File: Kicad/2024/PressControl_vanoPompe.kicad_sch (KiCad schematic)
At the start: 27 parts, among them J1 Conn_01x08_Pin, J2 Conn_01x08_Socket, J5 Conn_01x08_Socket, J6 Conn_01x08_Pin, K1 sOnOff_ClearContacts, P1 Pump, P2 Press_Control, SW1 TestAlarm, SW2 pc_Button

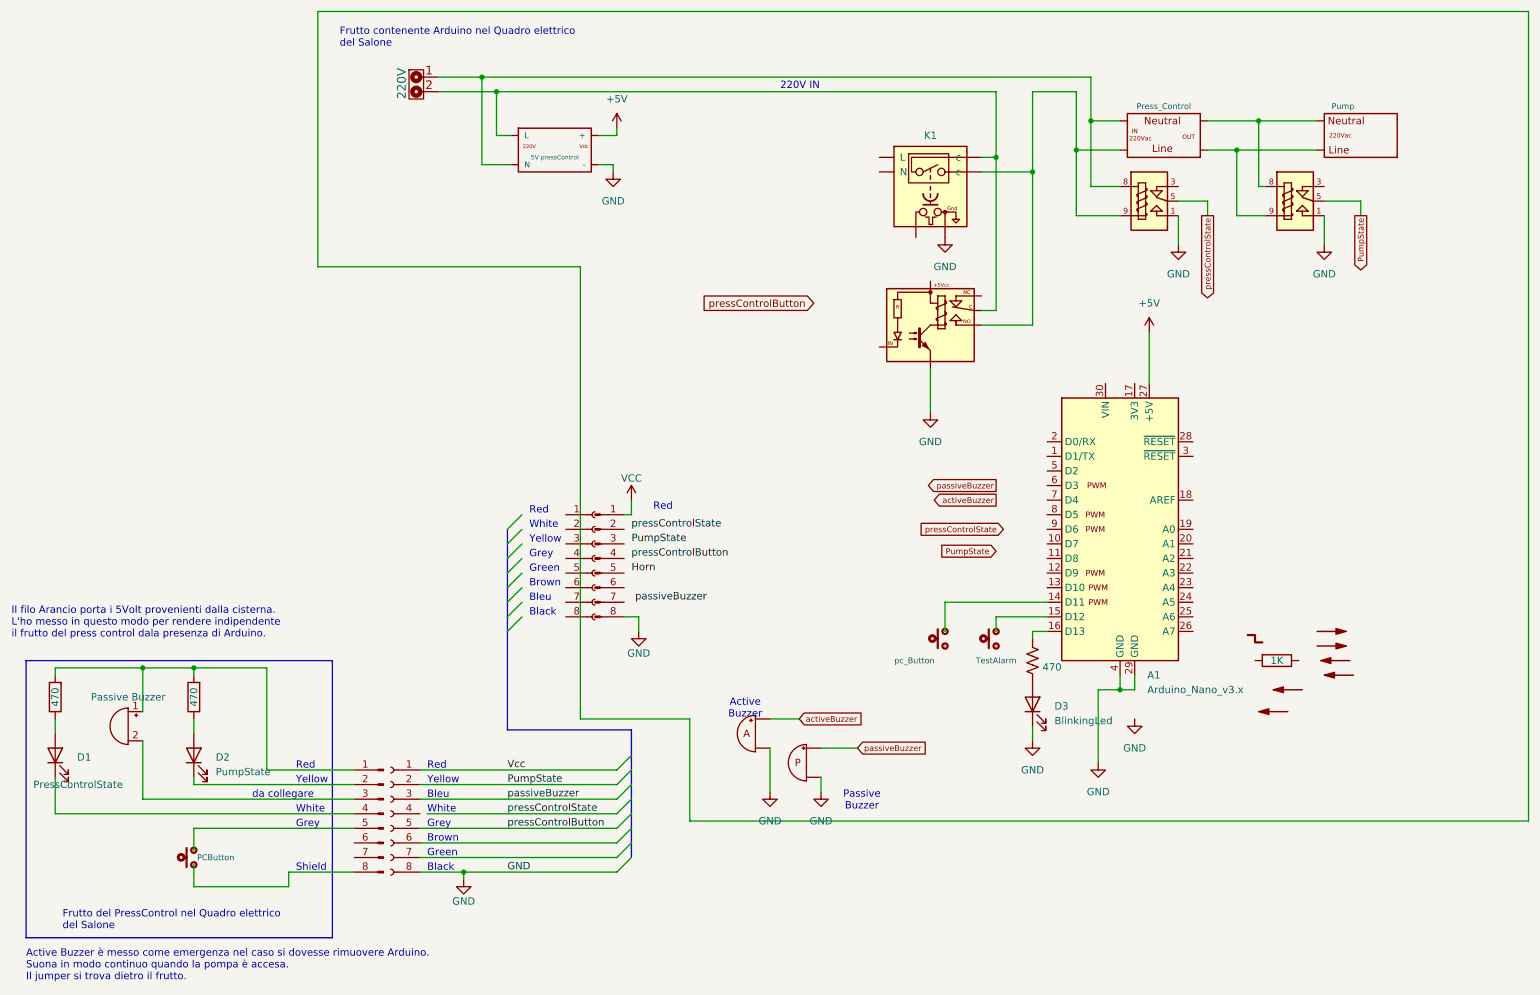
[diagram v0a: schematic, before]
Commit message: update
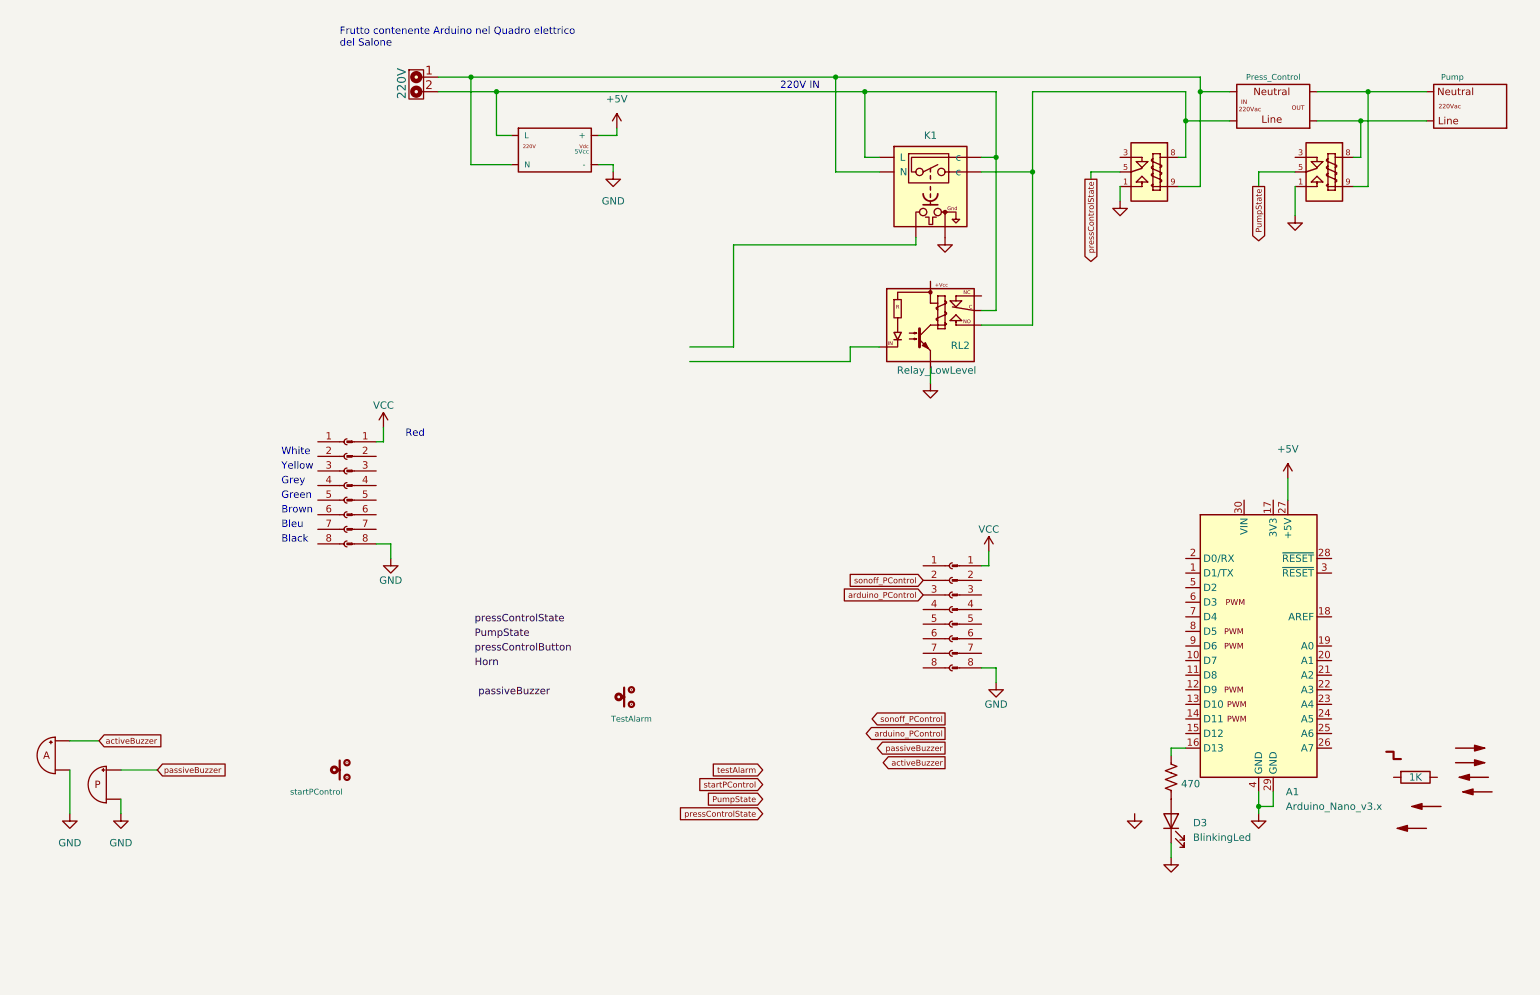
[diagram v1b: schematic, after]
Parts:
- removed BZ1: Passive Buzzer, symbol Device:Buzzer
- removed D1: PressControlState, symbol Device:LED
- removed D2: PumpState, symbol Device:LED
- removed J1: Conn_01x08_Pin, symbol Connector:Conn_01x08_Pin
- removed J2: Conn_01x08_Socket, symbol Connector:Conn_01x08_Socket
- removed R? (x2): 470, symbol Device:R
- removed RL1: Relay_5V_LL, symbol lnDevice:Relay_5V_LL
- removed SW?: PCButton, symbol LnDevice:PulsanteNO
- added J1: Conn_01x08_Socket, symbol Connector:Conn_01x08_Socket
- added J2: Conn_01x08_Pin, symbol Connector:Conn_01x08_Pin
- added RL2: Relay_LowLevel, symbol lnDevice:Relay_LowLevel
- Al_5Vcc?: footprint 5V pressControl -> 5Vcc
- SW2: value pc_Button -> startPControl
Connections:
- net GND: now also J2.8 (Pin_8), RL2.~
- net VCC: now also J2.1 (Pin_1)
- net at K?.8, P2.~ (2): now also K1. (c), RL2.~; no longer Al_5Vcc?.~ (N), J?.1
- net at SW1.2: no longer A1.15 (D12)
- net at A1.14 (D11): no longer SW2.2
- new net: Al_5Vcc?.~ (N), J?.1, K1. (c), K?.9, P2.~ (2)
- new net: Al_5Vcc?.~ (N), J?.2, K1. (c), RL2.~
- new net: K?.8, P1.~ (2), P2.~ (2)
- new net arduino_PControl: J1.3 (Pin_3)
- new net sonoff_PControl: J1.2 (Pin_2)
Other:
- note removed: "Active Buzzer"
- note removed: "Active Buzzer è messo come emergenza nel caso si dovesse rimuovere Arduino. Suona in modo continuo quando la pompa è accesa. Il jumper si trova dietro il frutto."
- note removed: "Frutto del PressControl nel Quadro elettrico del Salone"
- note removed: "Il filo Arancio porta i 5Volt provenienti dalla cisterna. L'ho messo in questo modo per rendere indipendente il frutto del press control dala presenza di Arduino."
- note removed: "Passive Buzzer"
- note removed: "Shield"
- note removed: "da collegare"
- moved on the sheet: A1, D3
